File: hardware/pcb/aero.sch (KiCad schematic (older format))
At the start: 0 parts

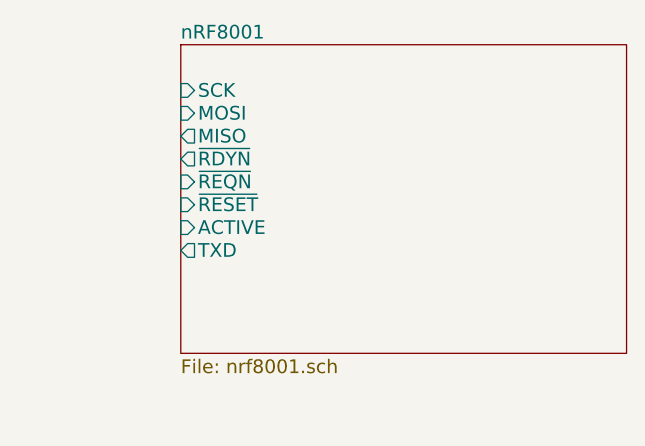
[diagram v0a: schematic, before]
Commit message: version 1 of layout
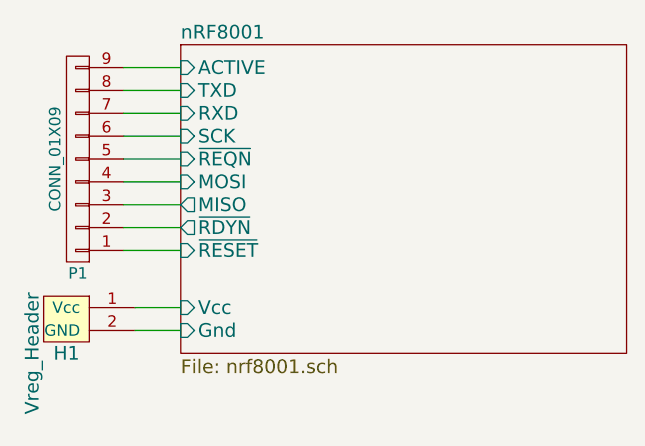
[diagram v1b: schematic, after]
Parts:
- added H1: Vreg_Header, Socket_Strips:Socket_Strip_Straight_1x02, symbol Vreg_Header
- added P1: CONN_01X09, Socket_Strips:Socket_Strip_Straight_1x09, symbol CONN_01X09
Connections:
- net nRF8001/ACTIVE: now also P1.9 (P9)
- net nRF8001/MISO: now also P1.3 (P3)
- net nRF8001/MOSI: now also P1.4 (P4)
- net nRF8001/SCK: now also P1.6 (P6)
- net nRF8001/TXD: now also P1.8 (P8)
- net nRF8001/~RDYN: now also P1.2 (P2)
- net nRF8001/~REQN: now also P1.5 (P5)
- net nRF8001/~RESET: now also P1.1 (P1)
- new net nRF8001/Gnd: H1.2 (GND)
- new net nRF8001/RXD: P1.7 (P7)
- new net nRF8001/Vcc: H1.1 (Vcc)
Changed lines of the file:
@@
 LIBS:contrib
 LIBS:valves
+LIBS:aero-cache
 EELAYER 25 0
 EELAYER END
@@
 Comment4 ""
 $EndDescr
+$Comp
+L CONN_01X09 P1
+U 1 1 551C5BBD
+P 7550 1650
+F 0 "P1" H 7550 2150 50  0000 C CNN
+F 1 "CONN_01X09" V 7650 1650 50  0000 C CNN
+F 2 "Socket_Strips:Socket_Strip_Straight_1x09" H 7550 1650 60  0001 C CNN
+F 3 "" H 7550 1650 60  0000 C CNN
+	1    7550 1650
+	-1   0    0    1
+$EndComp
+$Comp
+L Vreg_Header H1
+U 1 1 551C5F7E
+P 7550 2450
+F 0 "H1" H 7500 2400 60  0000 C CNN
+F 1 "Vreg_Header" V 7350 2400 60  0000 C CNN
+F 2 "Socket_Strips:Socket_Strip_Straight_1x02" H 7550 2450 60  0001 C CNN
+F 3 "" H 7550 2450 60  0000 C CNN
+	1    7550 2450
+	1    0    0    -1
+$EndComp
+Wire Wire Line
+	7800 2300 8000 2300
+Wire Wire Line
+	8000 2400 7800 2400
 $Sheet
 S 8000 1150 1950 1350
@@
 F0 "nRF8001" 60
 F1 "nrf8001.sch" 60
-F2 "MOSI" I L 8000 1450 60
-F3 "MISO" O L 8000 1550 60
-F4 "~RDYN" O L 8000 1650 60
-F5 "~REQN" I L 8000 1750 60
-F6 "SCK" I L 8000 1350 60
-F7 "~RESET" I L 8000 1850 60
-F8 "ACTIVE" I L 8000 1950 60
-F9 "TXD" O L 8000 2050 60
+F2 "Vcc" I L 8000 2300 60
+F3 "Gnd" I L 8000 2400 60
+F4 "MOSI" I L 8000 1750 60
+F5 "MISO" O L 8000 1850 60
+F6 "~RDYN" O L 8000 1950 60
+F7 "~REQN" I L 8000 1650 60
+F8 "SCK" I L 8000 1550 60
+F9 "~RESET" I L 8000 2050 60
+F10 "ACTIVE" I L 8000 1250 60
+F11 "TXD" I L 8000 1350 60
+F12 "RXD" I L 8000 1450 60
 $EndSheet
+Wire Wire Line
+	7750 1250 8000 1250
+Wire Wire Line
+	8000 1350 7750 1350
+Wire Wire Line
+	7750 1450 8000 1450
+Wire Wire Line
+	8000 1550 7750 1550
+Wire Wire Line
+	8000 1650 7750 1650
+Wire Wire Line
+	7750 1750 8000 1750
+Wire Wire Line
+	8000 1850 7750 1850
+Wire Wire Line
+	7750 1950 8000 1950
+Wire Wire Line
+	8000 2050 7750 2050
 $EndSCHEMATC
